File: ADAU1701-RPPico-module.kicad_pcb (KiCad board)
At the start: 4 copper layers, 100 x 100 mm, 92 parts, among them J1 Conn_01x04, J10 THONKICONN, J11 Conn_01x04, J2 Conn_01x04, J3 Conn_01x03, J4 Conn_01x02, J5 THONKICONN, J6 THONKICONN, J7 THONKICONN, J8 THONKICONN, J9 THONKICONN, U1 ADAU1701, U2 MCP1703A-3302_SOT23, U3 TL072, U4 TL074, U5 TL074, Y1 12.288MHz

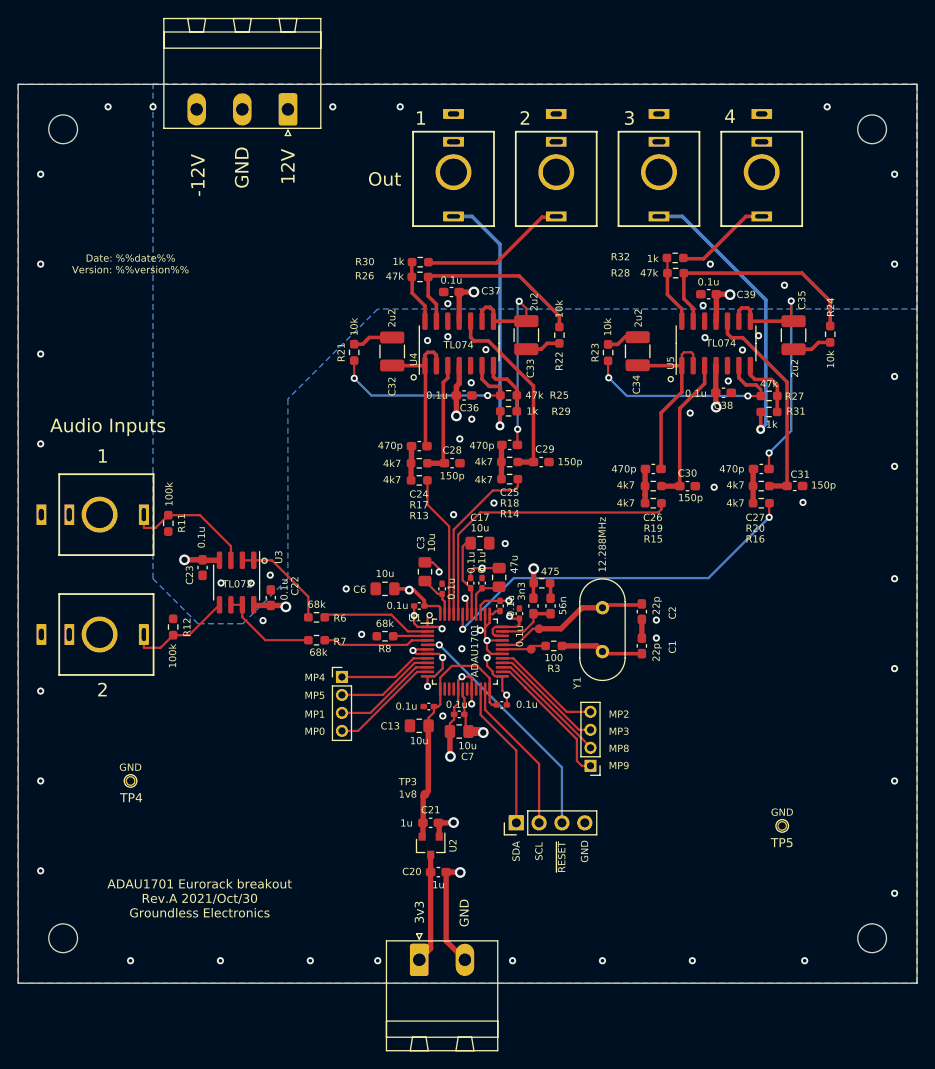
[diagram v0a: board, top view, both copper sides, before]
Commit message: Rev. B
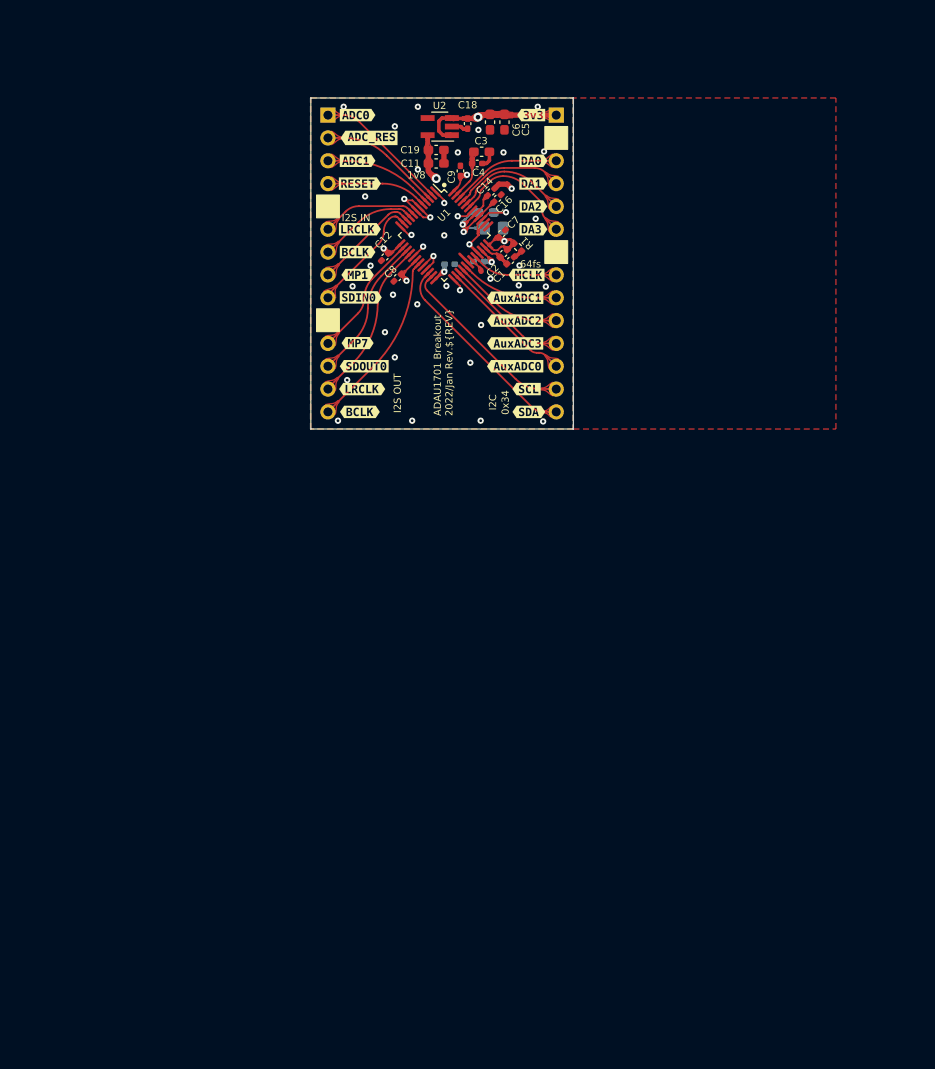
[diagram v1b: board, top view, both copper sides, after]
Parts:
- removed C20, C21: 1u, Capacitor_SMD:C_0603_1608Metric_Pad1.08x0.95mm_HandSolder
- removed C22, C23, C36, C37, C38, C39: 0.1u, Capacitor_SMD:C_0603_1608Metric_Pad1.08x0.95mm_HandSolder
- removed C24, C25, C26, C27: 470p, Capacitor_SMD:C_0603_1608Metric_Pad1.08x0.95mm_HandSolder
- removed C28, C29, C30, C31: 150p, Capacitor_SMD:C_0603_1608Metric_Pad1.08x0.95mm_HandSolder
- removed C32, C33, C34, C35: 2u2, Capacitor_SMD:C_1210_3225Metric_Pad1.33x2.70mm_HandSolder
- removed H1, H2, H3, H4: MountingHole, MountingHole:MountingHole_3.2mm_M3
- removed J10, J5, J6, J7, J8, J9: THONKICONN, Akiyuki_Footprint:THONKICONN
- removed J11: Conn_01x04, Connector_PinHeader_2.00mm:PinHeader_1x04_P2.00mm_Vertical
- removed J3: Conn_01x03, Connector_Phoenix_MSTB:PhoenixContact_MSTBA_2,5_3-G-5,08_1x03_P5.08mm_Horizontal
- removed J4: Conn_01x02, Connector_Phoenix_MSTB:PhoenixContact_MSTBA_2,5_2-G-5,08_1x02_P5.08mm_Horizontal
- removed R10: 475, Resistor_SMD:R_0603_1608Metric_Pad0.98x0.95mm_HandSolder
- removed R11, R12: 100k, Resistor_SMD:R_0603_1608Metric_Pad0.98x0.95mm_HandSolder
- removed R13, R14, R15, R16, R17, R18, R19, R20: 4k7, Resistor_SMD:R_0603_1608Metric_Pad0.98x0.95mm_HandSolder
- removed R21, R22, R23, R24: 10k, Resistor_SMD:R_0603_1608Metric_Pad0.98x0.95mm_HandSolder
- removed R25, R26, R27, R28: 47k, Resistor_SMD:R_0603_1608Metric_Pad0.98x0.95mm_HandSolder
- removed R29, R30, R31, R32: 1k, Resistor_SMD:R_0603_1608Metric_Pad0.98x0.95mm_HandSolder
- removed R3: 100, Resistor_SMD:R_0603_1608Metric_Pad0.98x0.95mm_HandSolder
- removed R6, R7, R8: 68k, Resistor_SMD:R_0603_1608Metric_Pad0.98x0.95mm_HandSolder
- removed TP3: TestPoint, Akiyuki_Footprint:TestPin_1.0SMD
- removed TP4, TP5: TestPoint, Akiyuki_Footprint:TestPin_0.8THT
- removed U3: TL072, Package_SO:SOIC-8_3.9x4.9mm_P1.27mm
- removed U4, U5: TL074, Package_SO:SOIC-14_3.9x8.7mm_P1.27mm
- removed Y1: 12.288MHz, Crystal:Crystal_HC49-U_Vertical
- added R1: 475, Resistor_SMD:R_0402_1005Metric_Pad0.72x0.64mm_HandSolder, F.Cu at (145.6, 73.1)
- added kibuzzard-61DAB0B4: G***, kibuzzard-61DAB0B4, F.Cu at (146.6, 76.2)
- added kibuzzard-61DAD9D2: G***, kibuzzard-61DAD9D2, F.Cu at (146.6, 88.9)
- added kibuzzard-61DAD9F7: G***, kibuzzard-61DAD9F7, F.Cu at (146.8, 91.4)
- added kibuzzard-61DADAE1: G***, kibuzzard-61DADAE1, F.Cu at (128.3, 88.9)
- added kibuzzard-61DADAF6: G***, kibuzzard-61DADAF6, F.Cu at (128.0, 91.4)
- added kibuzzard-61DADCE9: G***, kibuzzard-61DADCE9, F.Cu at (127.8, 83.8)
- added kibuzzard-61DADCF9: G***, kibuzzard-61DADCF9, F.Cu at (127.8, 76.2)
- added kibuzzard-61DADD90: G***, kibuzzard-61DADD90, F.Cu at (127.8, 73.7)
- added kibuzzard-61DADDC6: G***, kibuzzard-61DADDC6, F.Cu at (128.0, 71.1)
- added kibuzzard-61DADDE3: G***, kibuzzard-61DADDE3, F.Cu at (127.8, 58.4)
- added kibuzzard-61DADDF1: G***, kibuzzard-61DADDF1, F.Cu at (127.8, 63.5)
- added kibuzzard-61DADE19: G***, kibuzzard-61DADE19, F.Cu at (129.0, 61.0)
- added kibuzzard-61DADE61: G***, kibuzzard-61DADE61, F.Cu at (128.0, 66.0)
- added kibuzzard-61DADEF7: G***, kibuzzard-61DADEF7, F.Cu at (147.1, 58.4)
- added kibuzzard-61DADF35: G***, kibuzzard-61DADF35, F.Cu at (145.3, 86.4)
- added kibuzzard-61DADF43: G***, kibuzzard-61DADF43, F.Cu at (145.3, 78.7)
- added kibuzzard-61DADF53: G***, kibuzzard-61DADF53, F.Cu at (145.3, 81.3)
- added kibuzzard-61DADF5F: G***, kibuzzard-61DADF5F, F.Cu at (145.3, 83.8)
- added kibuzzard-61DAE5BF: G***, kibuzzard-61DAE5BF, F.Cu at (147.3, 66.0)
- added kibuzzard-61DAE5CD: G***, kibuzzard-61DAE5CD, F.Cu at (147.3, 68.6)
- added kibuzzard-61DAE5D9: G***, kibuzzard-61DAE5D9, F.Cu at (147.3, 71.1)
- added kibuzzard-61DAE5E4: G***, kibuzzard-61DAE5E4, F.Cu at (147.3, 63.5)
- added kibuzzard-61DBECC0: G***, kibuzzard-61DBECC0, F.Cu at (128.1, 78.7)
- added kibuzzard-61DBECE5: G***, kibuzzard-61DBECE5, F.Cu at (128.5, 86.4)
- C1: value 22p -> 56n; footprint Capacitor_SMD:C_0603_1608Metric_Pad1.08x0.95mm_HandSolder -> Capacitor_SMD:C_0402_1005Metric_Pad0.74x0.62mm_HandSolder
- C10: moved to B.Cu
- C11: value 0.1u -> 10u; footprint Capacitor_SMD:C_0402_1005Metric_Pad0.74x0.62mm_HandSolder -> Capacitor_SMD:C_0603_1608Metric_Pad1.08x0.95mm_HandSolder
- C12: value 56n -> 0.1u; footprint Capacitor_SMD:C_0603_1608Metric_Pad1.08x0.95mm_HandSolder -> Capacitor_SMD:C_0402_1005Metric_Pad0.74x0.62mm_HandSolder
- C13: value 10u -> 0.1u; footprint Capacitor_SMD:C_0805_2012Metric_Pad1.18x1.45mm_HandSolder -> Capacitor_SMD:C_0402_1005Metric_Pad0.74x0.62mm_HandSolder; moved to B.Cu
- C15: value 0.1u -> 10u; footprint Capacitor_SMD:C_0402_1005Metric_Pad0.74x0.62mm_HandSolder -> Capacitor_SMD:C_0603_1608Metric_Pad1.08x0.95mm_HandSolder; moved to B.Cu
- C17: value 10u -> 47u; moved to B.Cu
- C19: value 47u -> 2u2; footprint Capacitor_SMD:C_0805_2012Metric_Pad1.18x1.45mm_HandSolder -> Capacitor_SMD:C_0603_1608Metric_Pad1.08x0.95mm_HandSolder
- C2: value 22p -> 3n3; footprint Capacitor_SMD:C_0603_1608Metric_Pad1.08x0.95mm_HandSolder -> Capacitor_SMD:C_0402_1005Metric_Pad0.74x0.62mm_HandSolder
- C3, C6: footprint Capacitor_SMD:C_0805_2012Metric_Pad1.18x1.45mm_HandSolder -> Capacitor_SMD:C_0603_1608Metric_Pad1.08x0.95mm_HandSolder
- C5: value 3n3 -> 10u
- C7: value 10u -> 0.1u; footprint Capacitor_SMD:C_0805_2012Metric_Pad1.18x1.45mm_HandSolder -> Capacitor_SMD:C_0402_1005Metric_Pad0.74x0.62mm_HandSolder
- J1: value Conn_01x04 -> Conn_01x14; footprint Connector_PinHeader_2.00mm:PinHeader_1x04_P2.00mm_Vertical -> Connector_PinHeader_2.54mm:PinHeader_1x14_P2.54mm_Vertical; moved to B.Cu
- J2: value Conn_01x04 -> Conn_01x14; footprint Connector_PinHeader_2.54mm:PinHeader_1x04_P2.54mm_Vertical -> Connector_PinHeader_2.54mm:PinHeader_1x14_P2.54mm_Vertical; moved to B.Cu
- TP1: value TestPoint -> OSCO; footprint Akiyuki_Footprint:TestPin_1.0SMD -> Akiyuki_Footprint:TestPin_0.6SMD
- TP2: value TestPoint -> 1v8; footprint Akiyuki_Footprint:TestPin_1.0SMD -> Akiyuki_Footprint:TestPin_0.6SMD
- U2: value MCP1703A-3302_SOT23 -> NJM12888; footprint Package_TO_SOT_SMD:SOT-23 -> Package_TO_SOT_SMD:SOT-23-5_HandSoldering
- moved U2 80.0 mm to (136.9, 59.7), turned to 180 degrees
- moved J2 78.9 mm to (149.9, 58.4), turned to 180 degrees
- moved J1 62.5 mm to (124.5, 58.4), turned to 180 degrees
- moved C11 61.3 mm to (136.5, 63.8)
- moved C14 57.7 mm to (142.6, 67.0), turned to -135 degrees
- moved C7 55.6 mm to (143.8, 71.6), turned to 45 degrees
- moved C15 54.8 mm to (142.1, 69.2)
- moved TP2 54.1 mm to (135.8, 64.9)
- moved C5 54.0 mm to (142.5, 59.2), turned to -90 degrees
- moved C6 53.6 mm to (144.1, 59.2), turned to -90 degrees
- moved C13 51.5 mm to (138.0, 75.0), turned to 180 degrees
- moved C18 51.1 mm to (140.0, 59.4)
- moved C9 49.7 mm to (139.2, 64.6)
- moved C19 48.1 mm to (136.5, 62.3), turned to 0 degrees
- moved C4 47.5 mm to (141.1, 63.8), turned to 180 degrees
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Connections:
- C1 pad 2: GND -> Net-(C1-Pad2)
- C11 pad 1: +3V3 -> GND
- C11 pad 2: GND -> +1V8
- C12 pad 1: PLL_LF -> GND
- C12 pad 2: Net-(C12-Pad2) -> +1V8
- C14 pad 2: +1V8 -> Net-(C14-Pad2)
- C15 pad 2: +1V8 -> Net-(C14-Pad2)
- C18 pad 1: GND -> +3V3
- C18 pad 2: Net-(C18-Pad2) -> GND
- C19 pad 1: GND -> +1V8
- C19 pad 2: Net-(C18-Pad2) -> GND
- C2 pad 1: Net-(C2-Pad1) -> Net-(C1-Pad1)
- C2 pad 2: GND -> +3V3
- C5 pad 1: PLL_LF -> +3V3
- C5 pad 2: +3V3 -> GND
- J1 pad 1: MP4 -> /1701_ADC0
- J1 pad 2: MP5 -> /1701_ADC_RES
- J1 pad 3: MP1 -> /1701_ADC1
- J1 pad 4: MP0 -> /~{RESET}
- J2 pad 1: SDA -> +3V3
- J2 pad 2: SCL -> GND
- J2 pad 3: ~RESET -> /1701_VOUT0
- J2 pad 4: GND -> /1701_VOUT1
- TP1 pad 1: Net-(C2-Pad1) -> Net-(TP1-Pad1)
- TP2 pad 1: Net-(R3-Pad1) -> +1V8
- U1 pad 10: MP1 -> 1701_MP1
- U1 pad 11: MP0 -> 1701_In_SDIN0
- U1 pad 14: (no net) -> 1701_MP7
- U1 pad 15: (no net) -> 1701_Out_SDOUT0
- U1 pad 16: (no net) -> 1701_Out_LRCLK
- U1 pad 19: (no net) -> 1701_Out_BCLK
- U1 pad 2: Net-(R6-Pad1) -> /1701_ADC0
- U1 pad 21: (no net) -> GND
- U1 pad 22: SDA -> /SDA
- U1 pad 23: SCL -> /SCL
- U1 pad 26: MP9 -> 1701_AuxADC0
- U1 pad 27: MP8 -> 1701_AuxADC3
- U1 pad 28: MP3 -> 1701_AuxADC2
- U1 pad 29: MP2 -> 1701_AuxADC1
- U1 pad 3: Net-(R8-Pad1) -> /1701_ADC_RES
- U1 pad 31: Net-(R3-Pad1) -> Net-(TP1-Pad1)
- U1 pad 32: Net-(C2-Pad1) -> MCLK_In
- U1 pad 35: PLL_LF -> Net-(C1-Pad1)
- U1 pad 39: +3V3 -> GND
- U1 pad 4: Net-(R7-Pad1) -> /1701_ADC1
- U1 pad 40: Net-(C18-Pad2) -> Net-(C16-Pad2)
- U1 pad 41: Net-(C16-Pad2) -> Net-(C14-Pad2)
- U1 pad 43: DAC3 -> /1701_VOUT3
- U1 pad 44: DAC2 -> /1701_VOUT2
- U1 pad 45: DAC1 -> /1701_VOUT1
- U1 pad 46: DAC0 -> /1701_VOUT0
- U1 pad 5: ~RESET -> /~{RESET}
- U1 pad 8: MP4 -> 1701_In_LRCLK
- U1 pad 9: MP5 -> 1701_In_BCLK
- U2 pad 1: GND -> +3V3
- U2 pad 2: +1V8 -> GND
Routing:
- net DAC3: track 42.5 -> 0.00 mm, vias 2 -> 0
- net GND: track 72.7 -> 38.3 mm, vias 74 -> 41
- net DAC2: track 33.3 -> 0.00 mm
- net Net-(J9-Pad3): track 32.4 -> 0.00 mm, vias 1 -> 0
- net Net-(C27-Pad1): track 30.7 -> 0.00 mm, vias 2 -> 0
- net Net-(J7-Pad3): track 28.4 -> 0.00 mm, vias 1 -> 0
- net ~RESET: track 26.8 -> 0.00 mm, vias 1 -> 0
- net Net-(R24-Pad1): track 26.5 -> 0.00 mm
- net Net-(C25-Pad1): track 26.2 -> 0.00 mm, vias 2 -> 0
- net Net-(R23-Pad1): track 25.2 -> 0.00 mm, vias 2 -> 0
- net Net-(R21-Pad1): track 25.0 -> 0.00 mm, vias 2 -> 0
- net Net-(C31-Pad1): track 23.8 -> 0.00 mm
- net /SDA: track 0.00 -> 23.1 mm
- net Net-(R22-Pad1): track 23.0 -> 0.00 mm
- net Net-(C29-Pad1): track 21.7 -> 0.00 mm
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- added copper zone on In2.Cu, net +1V8
- removed copper zone on In2.Cu, net +12V
- removed copper zone on B.Cu, net -12V
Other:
- board size 100 x 100 mm -> 29.2 x 36.8 mm
- net class Default removed
- board text added: "0x34"
- board text added: "64fs"
- board text added: "ADAU1701 Breakout 2022/Jan Rev.${REV}"
- board text added: "I2C"
- board text added: "I2S IN"
- board text added: "I2S OUT"
- board text added: "JLCJLCJLCJLC"
- board text removed: "-12V"
- board text removed: "1"
- board text removed: "12V"
- board text removed: "1v8"
- board text removed: "2"
- board text removed: "3"
- board text removed: "3v3"
- board text removed: "4"
- board text removed: "ADAU1701 Eurorack breakout Rev.A 2021/Oct/30 Groundless Electronics"
- board text removed: "Audio Inputs"
- board text removed: "Date: %%date%% Version: %%version%%"
- board text removed: "GND"
- board text removed: "MP0"
- board text removed: "MP1"
- board text removed: "MP2"
- board text removed: "MP3"
- board text removed: "MP4"
- board text removed: "MP5"
- board text removed: "MP8"
- board text removed: "MP9"
- board text removed: "Out"
- board text removed: "SCL"
- board text removed: "SDA"
- board text removed: "~RESET"
